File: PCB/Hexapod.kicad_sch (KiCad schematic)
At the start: 11 parts, among them J1 Servo Driver In, J10 Out+, J2 Servo Driver Out, J3 Raspberry, J4 Servo Driver Out, J5 Servo Driver In, J6 Conn_02x06_Odd_Even, J7 IN-, J8 IN+, J9 Out-

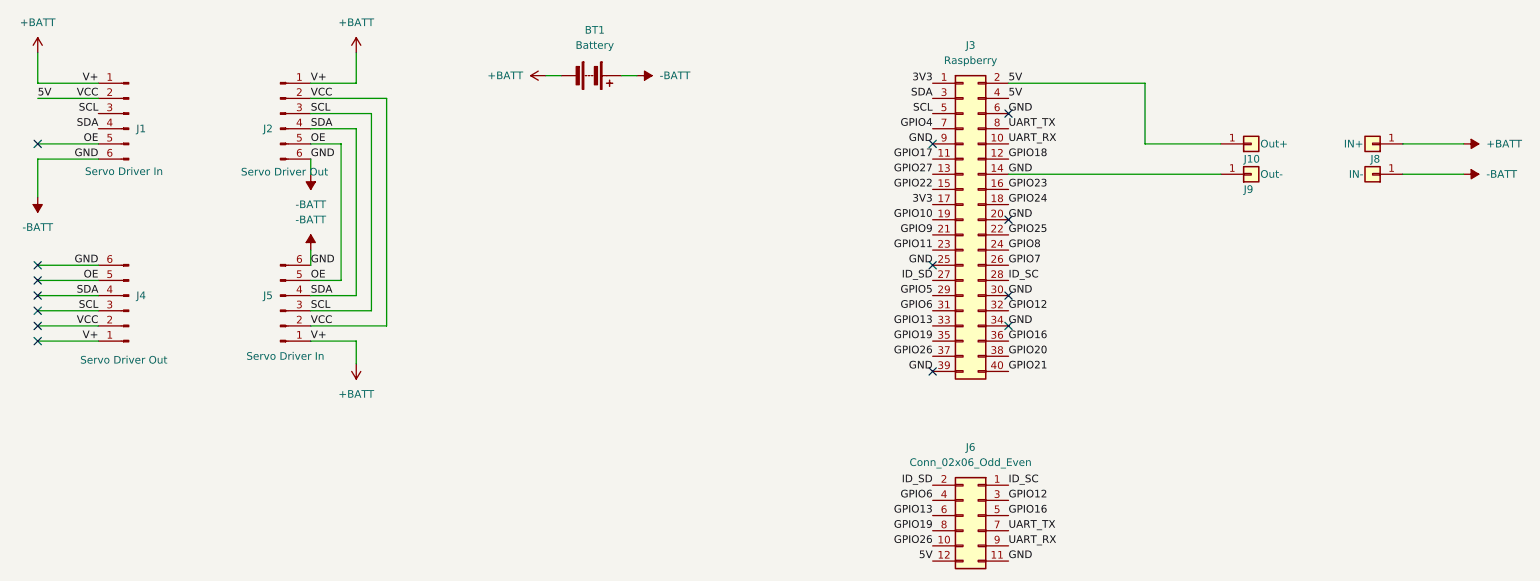
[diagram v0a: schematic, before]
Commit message: Update schematic and PCB
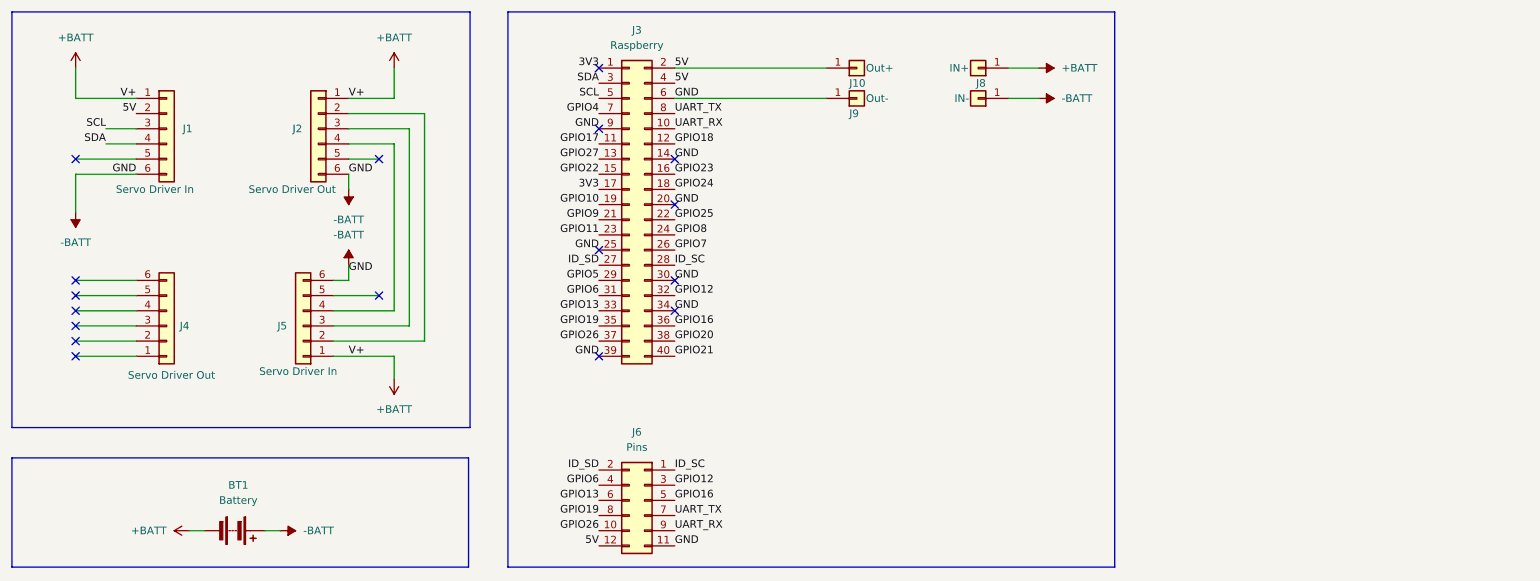
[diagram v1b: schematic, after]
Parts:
- J1, J2, J4, J5: symbol Connector:Conn_01x06_Pin -> Connector_Generic:Conn_01x06
- J6: value Conn_02x06_Odd_Even -> Pins
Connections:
- net +BATT: no longer J4.1 (Pin_1)
- net -BATT: no longer J4.6 (Pin_6)
- net 5V: no longer J2.2 (Pin_2), J4.2 (Pin_2), J5.2 (Pin_2)
- net SCL: no longer J2.3 (Pin_3), J4.3 (Pin_3), J5.3 (Pin_3)
- net SDA: no longer J2.4 (Pin_4), J4.4 (Pin_4), J5.4 (Pin_4)
- removed net OE: J1.5 (Pin_5), J2.5 (Pin_5), J4.5 (Pin_5), J5.5 (Pin_5)
- new net: J2.2 (Pin_2), J5.2 (Pin_2)
- new net: J2.3 (Pin_3), J5.3 (Pin_3)
- new net: J2.4 (Pin_4), J5.4 (Pin_4)
- no-connect marks 14 -> 17
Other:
- moved on the sheet: BT1, J10, J3, J6, J8, J9
